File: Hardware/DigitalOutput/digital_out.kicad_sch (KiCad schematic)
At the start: 40 parts, among them Q10 SI2347DS, Q11 SI2347DS, Q12 SI2347DS, Q13 SI2347DS, Q14 SI2347DS, Q15 SI2347DS, Q16 SI2347DS, Q9 SI2347DS, U10 CNY17-3, U11 CNY17-3, U12 CNY17-3, U13 CNY17-3, U14 CNY17-3, U15 CNY17-3, U16 CNY17-3, U9 CNY17-3

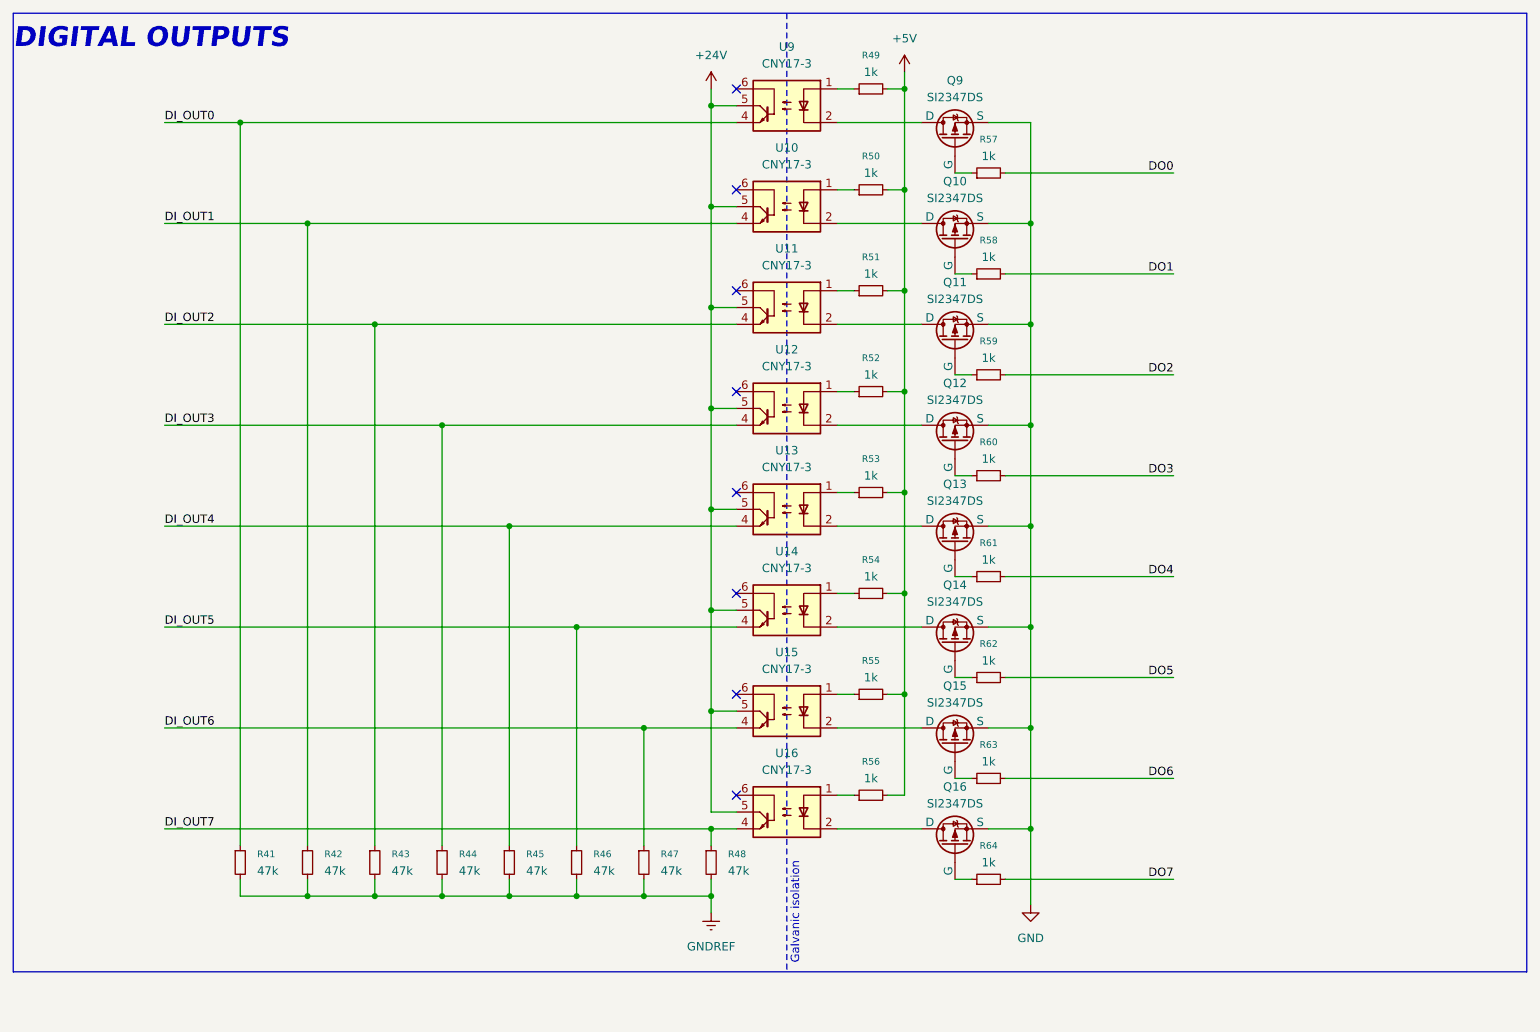
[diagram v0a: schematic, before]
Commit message: digital output & power finished
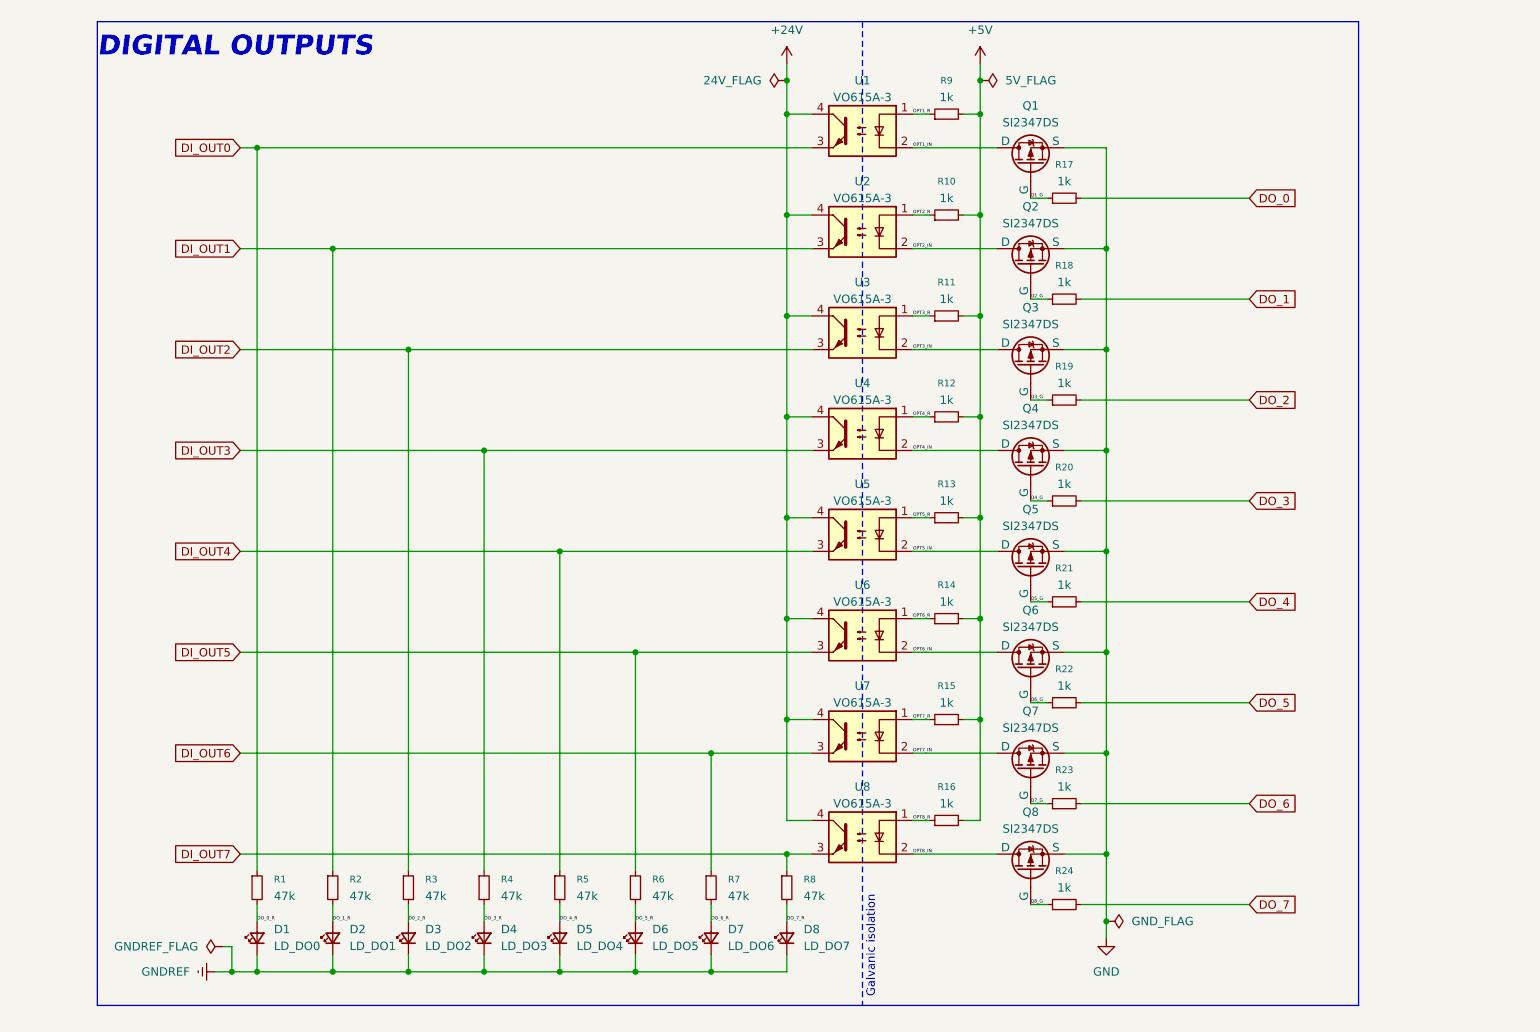
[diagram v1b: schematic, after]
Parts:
- removed U10, U11, U12, U13, U14, U15, U16, U9: CNY17-3, PLC_STM:SOP254P1016X400-6N, symbol Isolator:CNY17-3
- added D1: LD_DO0, LED_SMD:LED_0603_1608Metric_Pad1.05x0.95mm_HandSolder, symbol Device:LED_Small
- added D2: LD_DO1, LED_SMD:LED_0603_1608Metric_Pad1.05x0.95mm_HandSolder, symbol Device:LED_Small
- added D3: LD_DO2, LED_SMD:LED_0603_1608Metric_Pad1.05x0.95mm_HandSolder, symbol Device:LED_Small
- added D4: LD_DO3, LED_SMD:LED_0603_1608Metric_Pad1.05x0.95mm_HandSolder, symbol Device:LED_Small
- added D5: LD_DO4, LED_SMD:LED_0603_1608Metric_Pad1.05x0.95mm_HandSolder, symbol Device:LED_Small
- added D6: LD_DO5, LED_SMD:LED_0603_1608Metric_Pad1.05x0.95mm_HandSolder, symbol Device:LED_Small
- added D7: LD_DO6, LED_SMD:LED_0603_1608Metric_Pad1.05x0.95mm_HandSolder, symbol Device:LED_Small
- added D8: LD_DO7, LED_SMD:LED_0603_1608Metric_Pad1.05x0.95mm_HandSolder, symbol Device:LED_Small
- added U1, U2, U3, U4, U5, U6, U7, U8: VO615A-3, Package_DIP:DIP-4_W8.89mm_SMDSocket_LongPads, symbol Isolator:VO615A-3
- renumbered Q9 to Q1, Q10 to Q2, Q11 to Q3, Q12 to Q4, Q13 to Q5, Q14 to Q6, Q15 to Q7, Q16 to Q8, R41 to R1, R50 to R10, R51 to R11, R52 to R12, R53 to R13, R54 to R14, R55 to R15, R56 to R16, R57 to R17, R58 to R18, R59 to R19, R42 to R2, R60 to R20, R61 to R21, R62 to R22, R63 to R23, R64 to R24, R43 to R3, R44 to R4, R45 to R5, R46 to R6, R47 to R7, R48 to R8, R49 to R9
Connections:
- net +24V: now also U1.4, U2.4, U3.4, U4.4, U5.4, U6.4, U7.4, U8.4
- net DI_OUT0: now also U1.3
- net DI_OUT1: now also U2.3
- net DI_OUT2: now also U3.3
- net DI_OUT3: now also U4.3
- net DI_OUT4: now also U5.3
- net DI_OUT5: now also U6.3
- net DI_OUT6: now also U7.3
- net DI_OUT7: now also U8.3
- net GNDREF: now also D1.1 (K), D2.1 (K), D3.1 (K), D4.1 (K), D5.1 (K), D6.1 (K), D7.1 (K), D8.1 (K); no longer R1.2, R2.2, R3.2, R4.2, R5.2, R6.2, R7.2, R8.2
- net OPT4_IN: now reaches Q4.1 (D)
- net OPT4_IN: now also U4.2
- net Q4_G: now reaches Q4.2 (G), R20.1
- net OPT7_IN: now reaches Q7.1 (D)
- net OPT7_IN: now also U7.2
- net Q7_G: now reaches Q7.2 (G), R23.1
- net OPT8_R: now reaches R16.1
- net OPT8_R: now also U8.1
- net OPT8_IN: now reaches Q8.1 (D)
- net OPT8_IN: now also U8.2
- net OPT3_R: now reaches R11.1
- net OPT3_R: now also U3.1
- net OPT3_IN: now reaches Q3.1 (D)
- net OPT3_IN: now also U3.2
- net OPT2_IN: now reaches Q2.1 (D)
- net OPT2_IN: now also U2.2
- net Q2_G: now reaches Q2.2 (G), R18.1
- net OPT1_R: now reaches R9.1
- net OPT1_R: now also U1.1
- net OPT1_IN: now reaches Q1.1 (D)
- net OPT1_IN: now also U1.2
- net Q3_G: now reaches Q3.2 (G), R19.1
- net OPT5_R: now reaches R13.1
- net OPT5_R: now also U5.1
- net Q1_G: now reaches Q1.2 (G), R17.1
- net OPT6_R: now reaches R14.1
- net OPT6_R: now also U6.1
- net OPT7_R: now reaches R15.1
- net OPT7_R: now also U7.1
- net OPT6_IN: now reaches Q6.1 (D)
- net OPT6_IN: now also U6.2
- net Q6_G: now reaches Q6.2 (G), R22.1
- net OPT2_R: now reaches R10.1
- net OPT2_R: now also U2.1
- net OPT5_IN: now reaches Q5.1 (D)
- net OPT5_IN: now also U5.2
- net Q5_G: now reaches Q5.2 (G), R21.1
- net OPT4_R: now reaches R12.1
- net OPT4_R: now also U4.1
- net Q8_G: now reaches Q8.2 (G), R24.1
- net DO0 renamed DO_0
- net DO1 renamed DO_1
- net DO2 renamed DO_2
- net DO3 renamed DO_3
- net DO4 renamed DO_4
- net DO5 renamed DO_5
- net DO6 renamed DO_6
- net DO7 renamed DO_7
- new net D0_2_R: D3.2 (A), R3.2
- new net DO_0_R: D1.2 (A), R1.2
- new net DO_1_R: D2.2 (A), R2.2
- new net DO_3_R: D4.2 (A), R4.2
- new net DO_4_R: D5.2 (A), R5.2
- new net DO_5_R: D6.2 (A), R6.2
- new net DO_6_R: D7.2 (A), R7.2
- new net DO_7_R: D8.2 (A), R8.2
- no-connect marks 8 -> 0
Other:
- moved on the sheet: Q1, Q2, Q3, Q4, Q5, Q6, Q7, Q8, R1, R10, R11, R12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
